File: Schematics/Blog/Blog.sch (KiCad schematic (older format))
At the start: 1 part, among them U1 74HC00

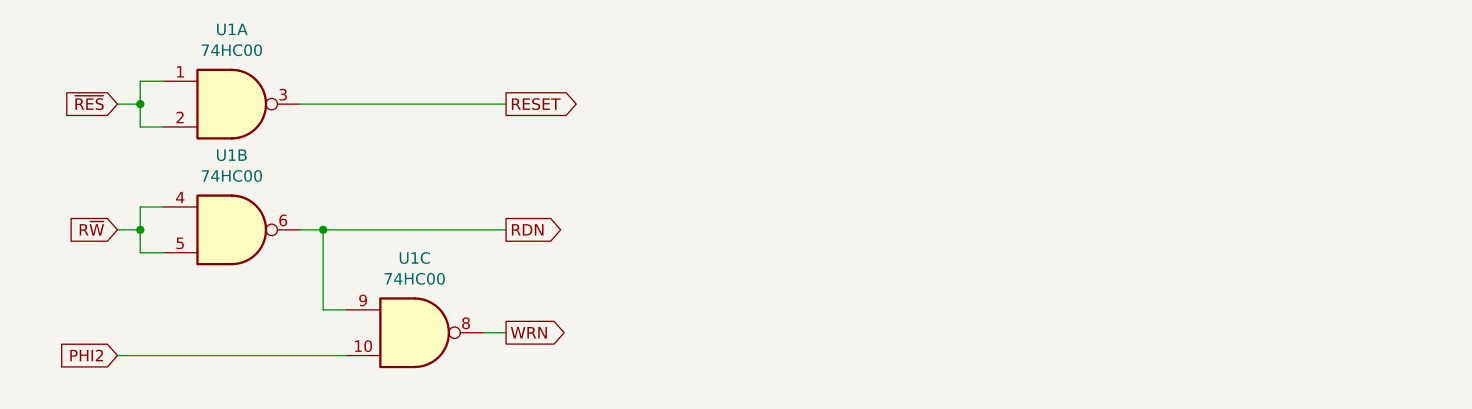
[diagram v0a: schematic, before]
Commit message: Started working on next article
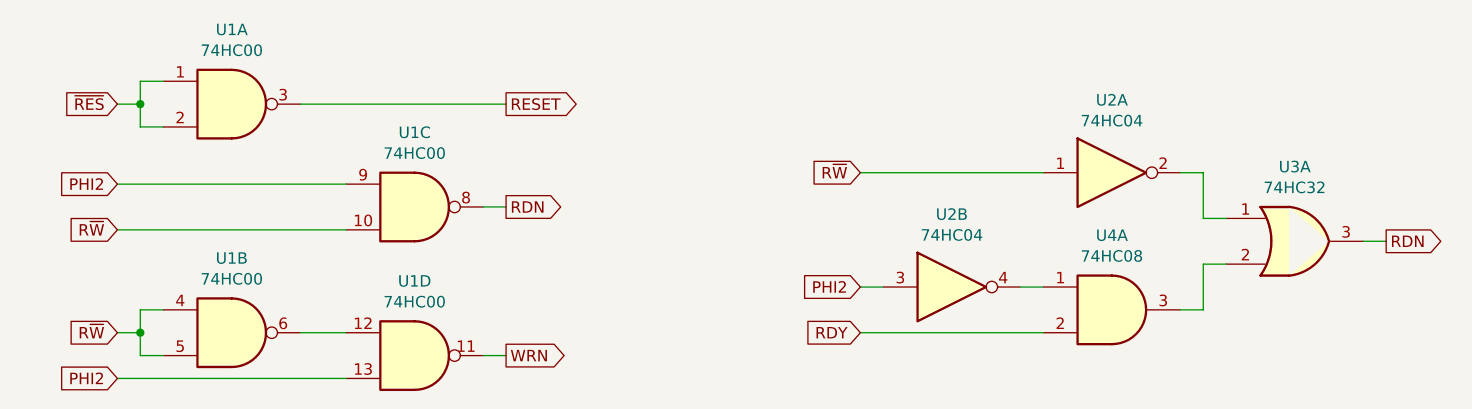
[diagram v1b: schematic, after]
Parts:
- added unit 3 of U1
- added U2: 74HC04, symbol 74xx:74HC04
- added U3: 74HC32, symbol 74xx:74LS32
- added U4: 74HC08, symbol 74xx:74LS08
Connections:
- net PHI2: now also U1.13, U1.9, U2.3; no longer U1.10
- net RDN: now also U1.8, U3.3; no longer U1.6, U1.9
- net R~W: now also U1.10, U2.1
- net WRN: now also U1.11; no longer U1.8
- new net: U1.12, U1.6
- new net: U2.2, U3.1
- new net: U3.2, U4.3
- new net: U2.4, U4.1
- new net RDY: U4.2
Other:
- moved on the sheet: U1B
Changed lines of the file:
@@
 L 74xx:74HC00 U1
 U 2 1 5FE31002
-P 2550 1850
-F 0 "U1" H 2550 2175 50  0000 C CNN
-F 1 "74HC00" H 2550 2084 50  0000 C CNN
-F 2 "" H 2550 1850 50  0001 C CNN
-F 3 "http://www.ti.com/lit/gpn/sn74hc00" H 2550 1850 50  0001 C CNN
-	2    2550 1850
+P 2550 2300
+F 0 "U1" H 2550 2625 50  0000 C CNN
+F 1 "74HC00" H 2550 2534 50  0000 C CNN
+F 2 "" H 2550 2300 50  0001 C CNN
+F 3 "http://www.ti.com/lit/gpn/sn74hc00" H 2550 2300 50  0001 C CNN
+	2    2550 2300
 	1    0    0    -1
 $EndComp
-Text GLabel 2050 1850 0    50   Input ~ 0
+Text GLabel 2050 2300 0    50   Input ~ 0
 R~W
 Wire Wire Line
-	2050 1850 2150 1850
+	2050 2300 2150 2300
 Wire Wire Line
-	2150 1850 2150 1950
+	2150 2300 2150 2400
 Wire Wire Line
-	2150 1950 2250 1950
+	2150 2400 2250 2400
 Wire Wire Line
-	2150 1850 2150 1750
+	2150 2300 2150 2200
 Wire Wire Line
-	2150 1750 2250 1750
-Connection ~ 2150 1850
-Text GLabel 3750 1850 2    50   Output ~ 0
+	2150 2200 2250 2200
+Connection ~ 2150 2300
+Text GLabel 3750 1750 2    50   Output ~ 0
 RDN
-Wire Wire Line
-	2850 1850 2950 1850
 $Comp
 L 74xx:74HC00 U1
-U 3 1 5FE3C714
-P 3350 2300
-F 0 "U1" H 3350 2625 50  0000 C CNN
-F 1 "74HC00" H 3350 2534 50  0000 C CNN
-F 2 "" H 3350 2300 50  0001 C CNN
-F 3 "http://www.ti.com/lit/gpn/sn74hc00" H 3350 2300 50  0001 C CNN
-	3    3350 2300
+U 4 1 5FE3C714
+P 3350 2400
+F 0 "U1" H 3350 2725 50  0000 C CNN
+F 1 "74HC00" H 3350 2634 50  0000 C CNN
+F 2 "" H 3350 2400 50  0001 C CNN
+F 3 "http://www.ti.com/lit/gpn/sn74hc00" H 3350 2400 50  0001 C CNN
+	4    3350 2400
+	1    0    0    -1
+$EndComp
+Text GLabel 3750 2400 2    50   Output ~ 0
+WRN
+Wire Wire Line
+	3650 2400 3750 2400
+Text GLabel 2050 2500 0    50   Input ~ 0
+PHI2
+Wire Wire Line
+	2050 2500 3050 2500
+$Comp
+L 74xx:74HC00 U1
+U 3 1 5FE4F41A
+P 3350 1750
+F 0 "U1" H 3350 2075 50  0000 C CNN
+F 1 "74HC00" H 3350 1984 50  0000 C CNN
+F 2 "" H 3350 1750 50  0001 C CNN
+F 3 "http://www.ti.com/lit/gpn/sn74hc00" H 3350 1750 50  0001 C CNN
+	3    3350 1750
 	1    0    0    -1
 $EndComp
 Wire Wire Line
-	2950 1850 2950 2200
+	3750 1750 3650 1750
 Wire Wire Line
-	2950 2200 3050 2200
+	2850 2300 3050 2300
 Wire Wire Line
-	2950 1850 3750 1850
-Connection ~ 2950 1850
-Text GLabel 3750 2300 2    50   Output ~ 0
-WRN
-Wire Wire Line
-	3650 2300 3750 2300
-Text GLabel 2050 2400 0    50   Input ~ 0
+	2050 1850 3050 1850
+Text GLabel 2050 1850 0    50   Input ~ 0
+R~W
+Text GLabel 2050 1650 0    50   Input ~ 0
 PHI2
 Wire Wire Line
-	2050 2400 3050 2400
+	2050 1650 3050 1650
+$Comp
+L 74xx:74LS32 U3
+U 1 1 5FE8D741
+P 7200 1900
+F 0 "U3" H 7200 2225 50  0000 C CNN
+F 1 "74HC32" H 7200 2134 50  0000 C CNN
+F 2 "" H 7200 1900 50  0001 C CNN
+F 3 "http://www.ti.com/lit/gpn/sn74LS32" H 7200 1900 50  0001 C CNN
+	1    7200 1900
+	1    0    0    -1
+$EndComp
+$Comp
+L 74xx:74HC04 U2
+U 1 1 5FE93B55
+P 6400 1600
+F 0 "U2" H 6400 1917 50  0000 C CNN
+F 1 "74HC04" H 6400 1826 50  0000 C CNN
+F 2 "" H 6400 1600 50  0001 C CNN
+F 3 "https://assets.nexperia.com/documents/data-sheet/74HC_HCT04.pdf" H 6400 1600 50  0001 C CNN
+	1    6400 1600
+	1    0    0    -1
+$EndComp
+Wire Wire Line
+	6700 1600 6800 1600
+Text GLabel 5300 1600 0    50   Input ~ 0
+R~W
+Wire Wire Line
+	5300 1600 6100 1600
+$Comp
+L 74xx:74HC04 U2
+U 2 1 5FE98581
+P 5700 2100
+F 0 "U2" H 5700 2417 50  0000 C CNN
+F 1 "74HC04" H 5700 2326 50  0000 C CNN
+F 2 "" H 5700 2100 50  0001 C CNN
+F 3 "https://assets.nexperia.com/documents/data-sheet/74HC_HCT04.pdf" H 5700 2100 50  0001 C CNN
+	2    5700 2100
+	1    0    0    -1
+$EndComp
+Text GLabel 5300 2100 0    50   Input ~ 0
+PHI2
+Wire Wire Line
+	5300 2100 5400 2100
+$Comp
+L 74xx:74LS08 U4
+U 1 1 5FE9F846
+P 6400 2200
+F 0 "U4" H 6400 2525 50  0000 C CNN
+F 1 "74HC08" H 6400 2434 50  0000 C CNN
+F 2 "" H 6400 2200 50  0001 C CNN
+F 3 "http://www.ti.com/lit/gpn/sn74LS08" H 6400 2200 50  0001 C CNN
+	1    6400 2200
+	1    0    0    -1
+$EndComp
+Wire Wire Line
+	6000 2100 6100 2100
+Text GLabel 5300 2300 0    50   Input ~ 0
+RDY
+Wire Wire Line
+	5300 2300 6100 2300
+Wire Wire Line
+	6700 2200 6800 2200
+Wire Wire Line
+	6800 2200 6800 2000
+Wire Wire Line
+	6800 2000 6900 2000
+Wire Wire Line
+	6800 1600 6800 1800
+Wire Wire Line
+	6800 1800 6900 1800
+Text GLabel 7600 1900 2    50   Output ~ 0
+RDN
+Wire Wire Line
+	7500 1900 7600 1900
 $EndSCHEMATC
